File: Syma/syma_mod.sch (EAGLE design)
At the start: 6 parts, among them Q1 BSS84, Q2 BSS84, Q3 BSS84

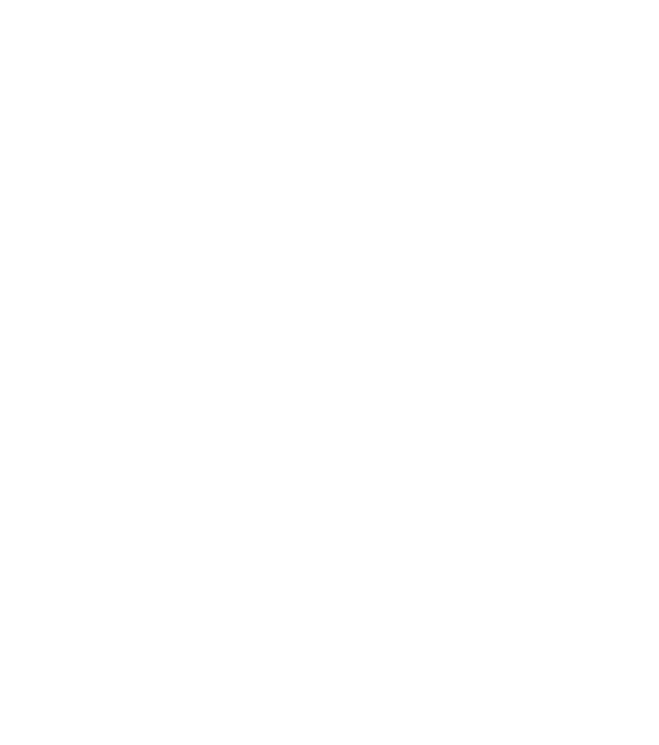
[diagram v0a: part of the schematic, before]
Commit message: syma update
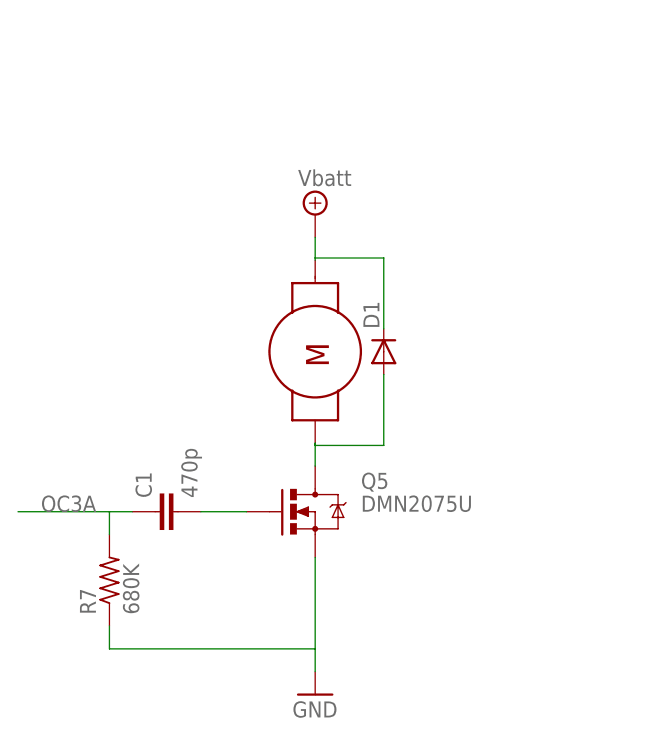
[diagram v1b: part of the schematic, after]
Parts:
- added C1: 470p, rcl:C-EUC0603
- added D1: (no value), palmquad_alpha:DIODE-MINIMELF
- added M4: MOTORARM-CORNER, palmquad_alpha:MOTORARM-CORNER
- added Q5: DMN2075U, palmquad_alpha:MOSFET-NCHANNELSMD
- added R7: 680K, rcl:R-US_R0603
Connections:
- new net GND: Q5.S, R7.1
- new net N$20: D1.A, M4.2, Q5.D
- new net N$45: C1.2, Q5.G
- new net OC3A: C1.1, R7.2
- new net VBATT: D1.C, M4.1
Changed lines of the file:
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@@
 <layer number="48" name="Document" color="7" fill="1" visible="no" active="no"/>
 <layer number="49" name="Reference" color="7" fill="1" visible="no" active="no"/>
+<layer number="50" name="dxf" color="7" fill="1" visible="no" active="no"/>
 <layer number="51" name="tDocu" color="7" fill="1" visible="no" active="no"/>
 <layer number="52" name="bDocu" color="7" fill="1" visible="no" active="no"/>
+<layer number="53" name="tGND_GNDA" color="7" fill="9" visible="no" active="no"/>
+<layer number="54" name="bGND_GNDA" color="1" fill="9" visible="no" active="no"/>
+<layer number="56" name="wert" color="7" fill="1" visible="no" active="no"/>
 <layer number="90" name="Modules" color="5" fill="1" visible="yes" active="yes"/>
 <layer number="91" name="Nets" color="2" fill="1" visible="yes" active="yes"/>
@@
 <layer number="97" name="Info" color="7" fill="1" visible="yes" active="yes"/>
 <layer number="98" name="Guide" color="6" fill="1" visible="yes" active="yes"/>
+<layer number="100" name="Muster" color="7" fill="1" visible="no" active="no"/>
+<layer number="101" name="Patch_Top" color="12" fill="4" visible="yes" active="yes"/>
+<layer number="102" name="Vscore" color="7" fill="1" visible="yes" active="yes"/>
+<layer number="103" name="tMap" color="7" fill="1" visible="yes" active="yes"/>
+<layer number="104" name="Name" color="16" fill="1" visible="yes" active="yes"/>
+<layer number="105" name="tPlate" color="7" fill="1" visible="yes" active="yes"/>
+<layer number="106" name="bPlate" color="7" fill="1" visible="yes" active="yes"/>
+<layer number="107" name="Crop" color="7" fill="1" visible="yes" active="yes"/>
+<layer number="116" name="Patch_BOT" color="9" fill="4" visible="yes" active="yes"/>
+<layer number="121" name="_tsilk" color="7" fill="1" visible="yes" active="yes"/>
+<layer number="122" name="_bsilk" color="7" fill="1" visible="yes" active="yes"/>
+<layer number="125" name="_tNames" color="7" fill="1" visible="no" active="yes"/>
+<layer number="144" name="Drill_legend" color="7" fill="1" visible="no" active="yes"/>
+<layer number="151" name="HeatSink" color="7" fill="1" visible="yes" active="yes"/>
+<layer number="200" name="200bmp" color="1" fill="10" visible="yes" active="yes"/>
+<layer number="201" name="201bmp" color="2" fill="10" visible="yes" active="yes"/>
+<layer number="202" name="202bmp" color="3" fill="10" visible="yes" active="yes"/>
+<layer number="203" name="203bmp" color="4" fill="10" visible="yes" active="yes"/>
+<layer number="204" name="204bmp" color="5" fill="10" visible="yes" active="yes"/>
+<layer number="205" name="205bmp" color="6" fill="10" visible="yes" active="yes"/>
+<layer number="206" name="206bmp" color="7" fill="10" visible="yes" active="yes"/>
+<layer number="207" name="207bmp" color="8" fill="10" visible="yes" active="yes"/>
+<layer number="208" name="208bmp" color="9" fill="10" visible="yes" active="yes"/>
+<layer number="209" name="209bmp" color="7" fill="1" visible="yes" active="yes"/>
+<layer number="210" name="210bmp" color="7" fill="1" visible="yes" active="yes"/>
+<layer number="211" name="211bmp" color="7" fill="1" visible="yes" active="yes"/>
+<layer number="212" name="212bmp" color="7" fill="1" visible="yes" active="yes"/>
+<layer number="213" name="213bmp" color="7" fill="1" visible="yes" active="yes"/>
+<layer number="214" name="214bmp" color="7" fill="1" visible="yes" active="yes"/>
+<layer number="215" name="215bmp" color="7" fill="1" visible="yes" active="yes"/>
+<layer number="216" name="216bmp" color="7" fill="1" visible="yes" active="yes"/>
+<layer number="217" name="217bmp" color="7" fill="1" visible="yes" active="yes"/>
+<layer number="218" name="218bmp" color="7" fill="1" visible="yes" active="yes"/>
+<layer number="219" name="219bmp" color="7" fill="1" visible="yes" active="yes"/>
+<layer number="220" name="220bmp" color="7" fill="1" visible="yes" active="yes"/>
+<layer number="221" name="221bmp" color="7" fill="1" visible="yes" active="yes"/>
+<layer number="222" name="222bmp" color="7" fill="1" visible="yes" active="yes"/>
+<layer number="223" name="223bmp" color="7" fill="1" visible="yes" active="yes"/>
+<layer number="224" name="224bmp" color="7" fill="1" visible="yes" active="yes"/>
+<layer number="250" name="Descript" color="3" fill="1" visible="no" active="no"/>
+<layer number="251" name="SMDround" color="12" fill="11" visible="no" active="no"/>
+<layer number="254" name="cooling" color="7" fill="1" visible="yes" active="yes"/>
 </layers>
 <schematic xreflabel="%F%N/%S.%C%R" xrefpart="/%S.%C%R">
@@
 </part>
 <part name="SUPPLY1" library="supply2" deviceset="GND" device=""/>
+<part name="M4" library="palmquad_alpha" deviceset="MOTOR" device="ARM-CORNER"/>
+<part name="Q5" library="palmquad_alpha" deviceset="MOSFET-NCHANNEL" device="SMD" value="DMN2075U"/>
+<part name="R7" library="rcl" deviceset="R-US_" device="R0603" value="680K"/>
+<part name="GND20" library="supply1" deviceset="GND" device=""/>
+<part name="SUPPLY8" library="supply2" deviceset="+5V" device="" value="Vbatt"/>
+<part name="D1" library="palmquad_alpha" deviceset="DIODE-" device="MINIMELF"/>
+<part name="C1" library="rcl" deviceset="C-EU" device="C0603" value="470p"/>
 </parts>
 <sheets>
@@
 </instance>
 <instance part="SUPPLY1" gate="GND" x="114.3" y="180.34"/>
+<instance part="M4" gate="G$1" x="83.82" y="83.82" rot="R270"/>
+<instance part="Q5" gate="G$1" x="83.82" y="66.04"/>
+<instance part="R7" gate="G$1" x="60.96" y="58.42" rot="R90"/>
+<instance part="GND20" gate="1" x="83.82" y="45.72"/>
+<instance part="SUPPLY8" gate="+5V" x="83.82" y="99.06"/>
+<instance part="D1" gate="G$1" x="91.44" y="83.82" rot="R90"/>
+<instance part="C1" gate="G$1" x="66.04" y="66.04" rot="R90"/>
 </instances>
 <busses>
@@
 <pinref part="SUPPLY1" gate="GND" pin="GND"/>
 </segment>
+<segment>
+<wire x1="83.82" y1="60.96" x2="83.82" y2="50.8" width="0.1524" layer="91"/>
+<wire x1="83.82" y1="50.8" x2="83.82" y2="48.26" width="0.1524" layer="91"/>
+<wire x1="60.96" y1="53.34" x2="60.96" y2="50.8" width="0.1524" layer="91"/>
+<wire x1="60.96" y1="50.8" x2="83.82" y2="50.8" width="0.1524" layer="91"/>
+<pinref part="Q5" gate="G$1" pin="S"/>
+<pinref part="GND20" gate="1" pin="GND"/>
+<pinref part="R7" gate="G$1" pin="1"/>
+</segment>
 </net>
 <net name="N$1" class="0">
@@
 </segment>
 </net>
+<net name="N$20" class="0">
+<segment>
+<wire x1="83.82" y1="73.66" x2="83.82" y2="71.12" width="0.1524" layer="91"/>
+<wire x1="83.82" y1="73.406" x2="83.82" y2="73.66" width="0.1524" layer="91"/>
+<wire x1="91.44" y1="81.28" x2="91.44" y2="73.406" width="0.1524" layer="91"/>
+<wire x1="91.44" y1="73.406" x2="83.82" y2="73.406" width="0.1524" layer="91"/>
+<pinref part="Q5" gate="G$1" pin="D"/>
+<pinref part="M4" gate="G$1" pin="2"/>
+<pinref part="D1" gate="G$1" pin="A"/>
+</segment>
+</net>
+<net name="OC3A" class="0">
+<segment>
+<wire x1="60.96" y1="66.04" x2="60.96" y2="63.5" width="0.1524" layer="91"/>
+<wire x1="60.96" y1="66.04" x2="50.8" y2="66.04" width="0.1524" layer="91"/>
+<wire x1="60.96" y1="66.04" x2="63.5" y2="66.04" width="0.1524" layer="91"/>
+<label x="53.34" y="66.04" size="1.778" layer="95"/>
+<pinref part="R7" gate="G$1" pin="2"/>
+<pinref part="C1" gate="G$1" pin="1"/>
+</segment>
+</net>
+<net name="VBATT" class="0">
+<segment>
+<wire x1="83.82" y1="96.52" x2="83.82" y2="94.234" width="0.1524" layer="91"/>
+<wire x1="83.82" y1="94.234" x2="83.82" y2="93.98" width="0.1524" layer="91"/>
+<wire x1="91.44" y1="86.36" x2="91.44" y2="94.234" width="0.1524" layer="91"/>
+<wire x1="91.44" y1="94.234" x2="83.82" y2="94.234" width="0.1524" layer="91"/>
+<pinref part="SUPPLY8" gate="+5V" pin="+5V"/>
+<pinref part="M4" gate="G$1" pin="1"/>
+<pinref part="D1" gate="G$1" pin="C"/>
+</segment>
+</net>
+<net name="N$45" class="0">
+<segment>
+<wire x1="71.12" y1="66.04" x2="76.2" y2="66.04" width="0.1524" layer="91"/>
+<pinref part="Q5" gate="G$1" pin="G"/>
+<pinref part="C1" gate="G$1" pin="2"/>
+</segment>
+</net>
